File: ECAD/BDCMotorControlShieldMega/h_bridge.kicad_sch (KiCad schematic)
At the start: 23 parts, among them J18 Motor Connector, J19 Limit switch, J8 Limit switch, U14 INA180A1, U7 DRV8870DDA

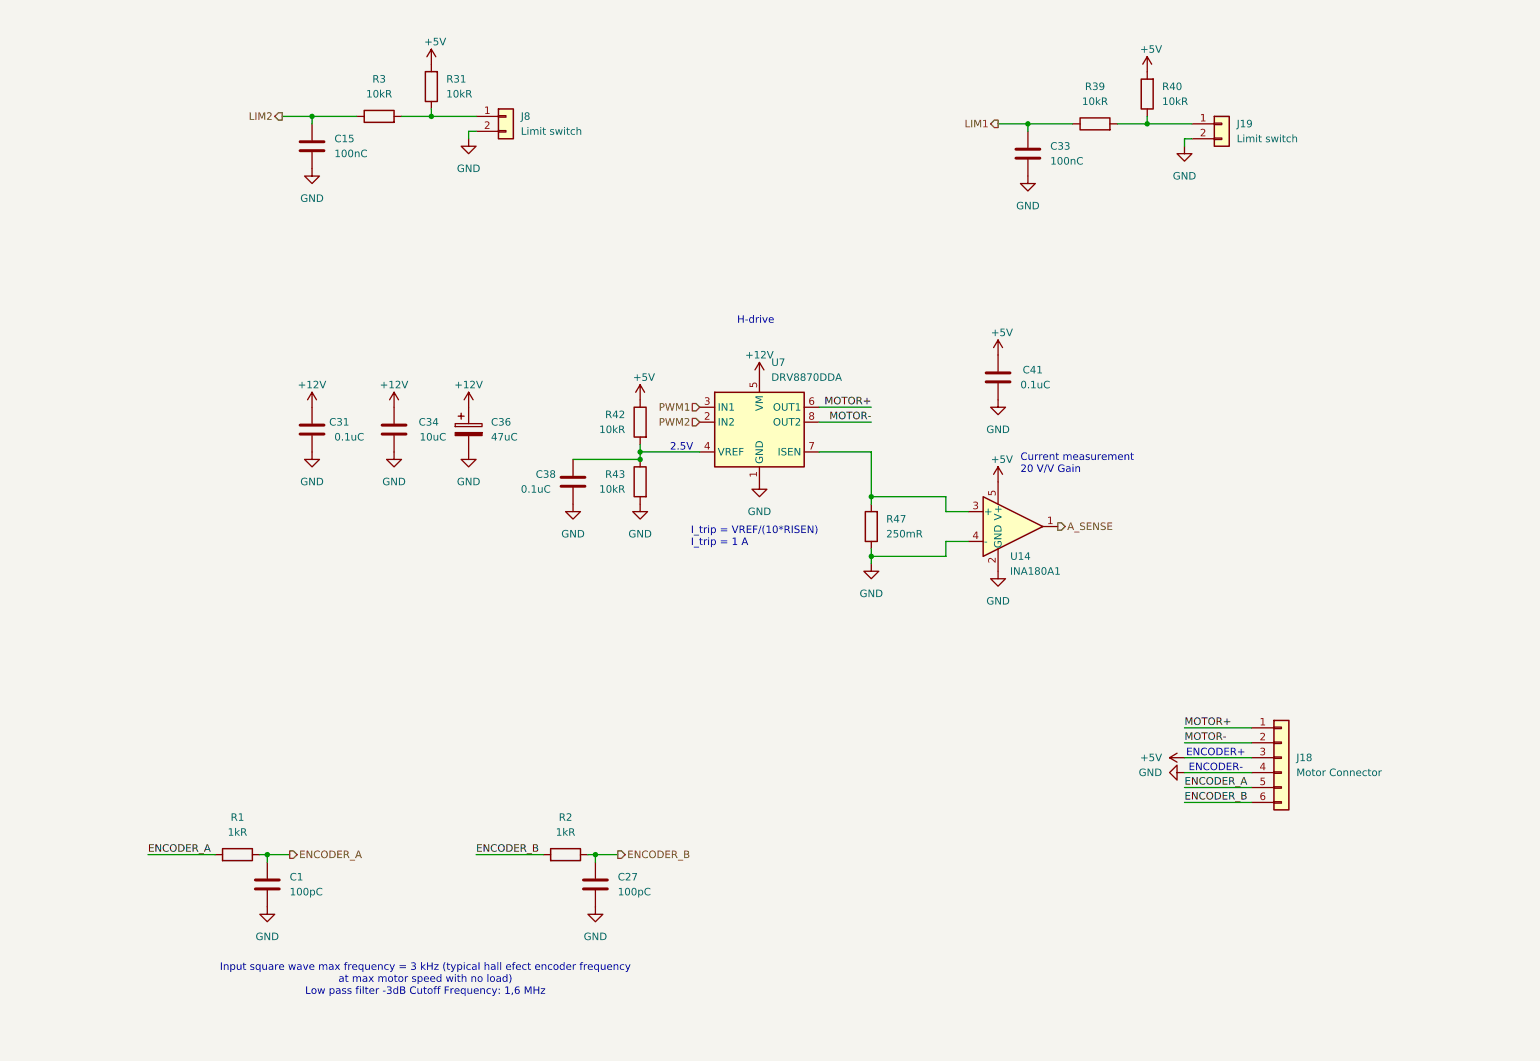
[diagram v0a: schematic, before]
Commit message: Progressed ECAD.
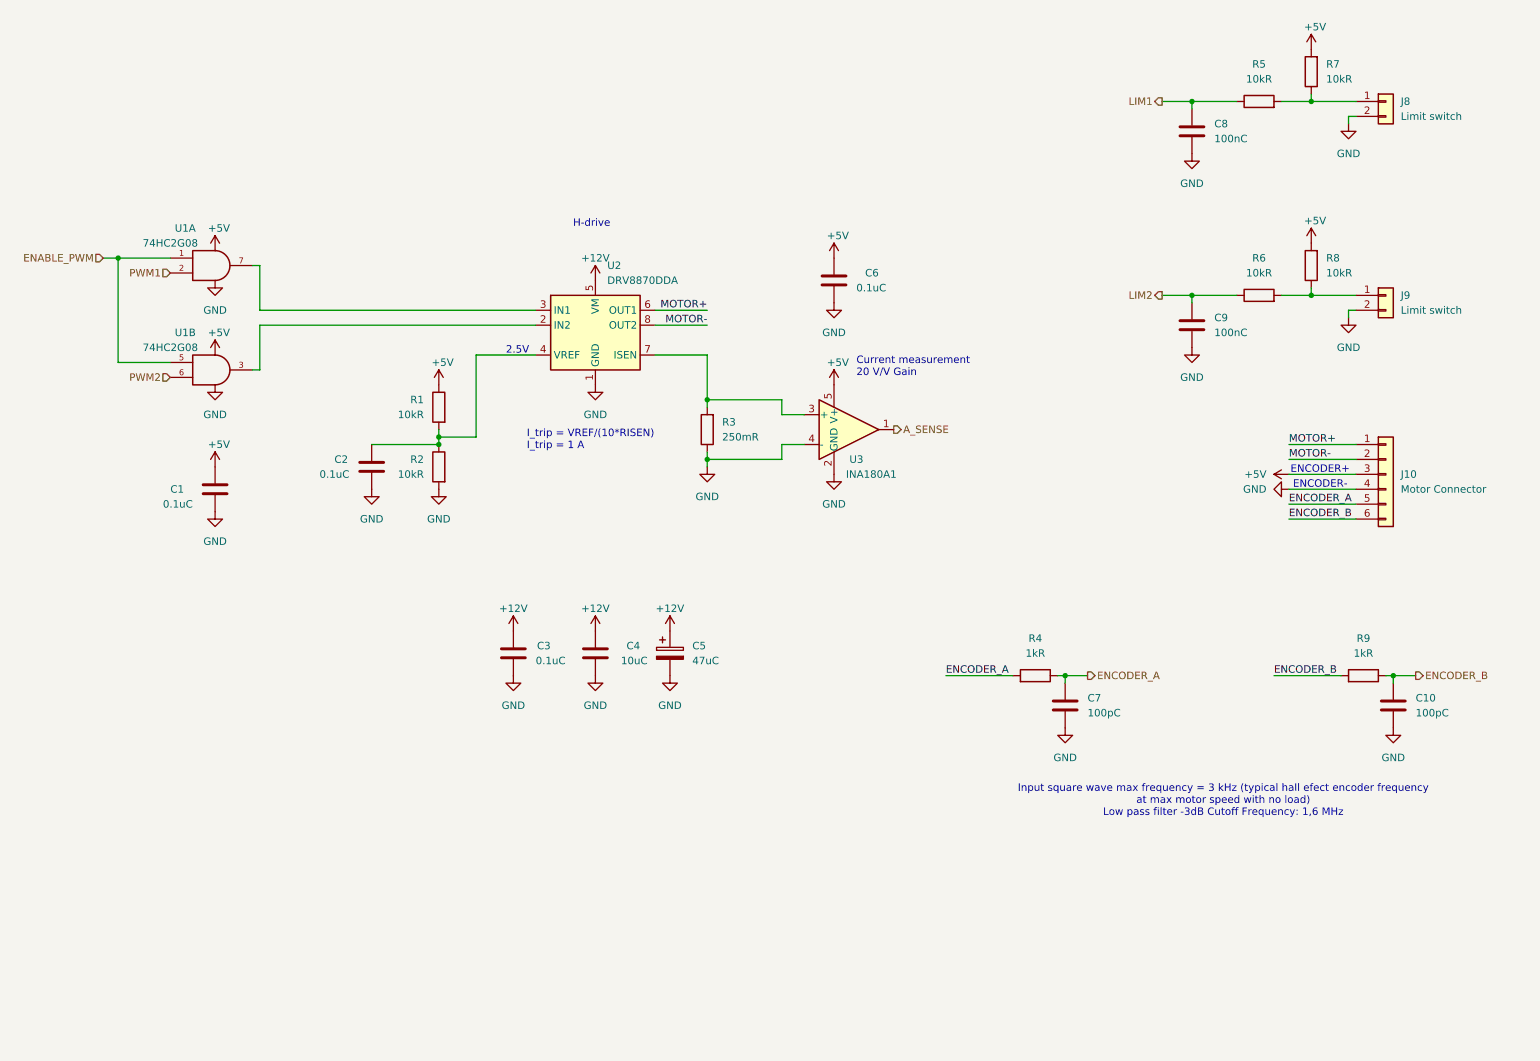
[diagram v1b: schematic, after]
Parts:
- added C1: 0.1uC, Capacitor_SMD:C_0805_2012Metric_Pad1.18x1.45mm_HandSolder, symbol Device:C
- added U1: 74HC2G08, Package_SO:TSSOP-8_3x3mm_P0.65mm, symbol 74xGxx:74LVC2G08
- renumbered C27 to C10, C38 to C2, C31 to C3, C34 to C4, C36 to C5, C41 to C6, C1 to C7, C33 to C8, C15 to C9, J18 to J10, J19 to J8, J8 to J9, R42 to R1, R43 to R2, R47 to R3, R1 to R4, R39 to R5, R3 to R6, R40 to R7, R31 to R8, R2 to R9, U7 to U2, U14 to U3
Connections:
- net +5V: now also C1.1, U1.8 (VCC), U1.8 (VCC)
- net GND: now also C1.2, U1.4 (GND), U1.4 (GND)
- net PWM1: now also U1.2; no longer U2.3 (IN1)
- net PWM2: now also U1.6; no longer U2.2 (IN2)
- new net: U1.3, U2.2 (IN2)
- new net: U1.7, U2.3 (IN1)
- new net ENABLE_PWM: U1.1, U1.5
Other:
- moved on the sheet: C10, C2, C3, C4, C5, C6, C7, C8, C9, J10, J8, J9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

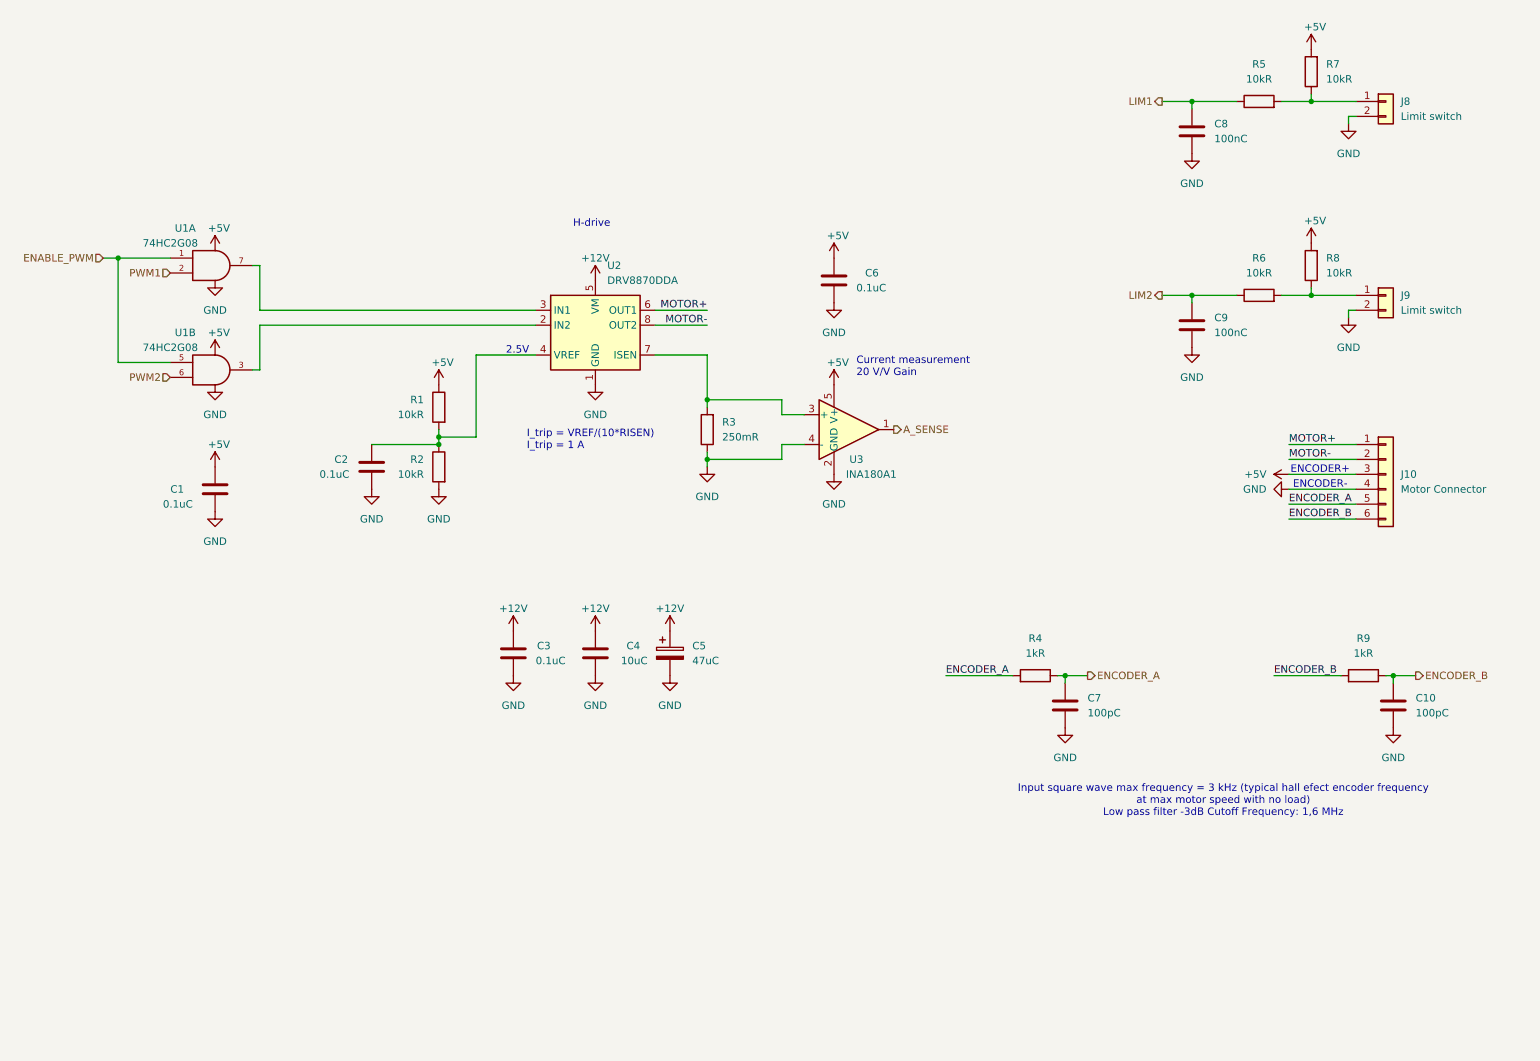
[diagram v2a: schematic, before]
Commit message: Progressed ECAD.
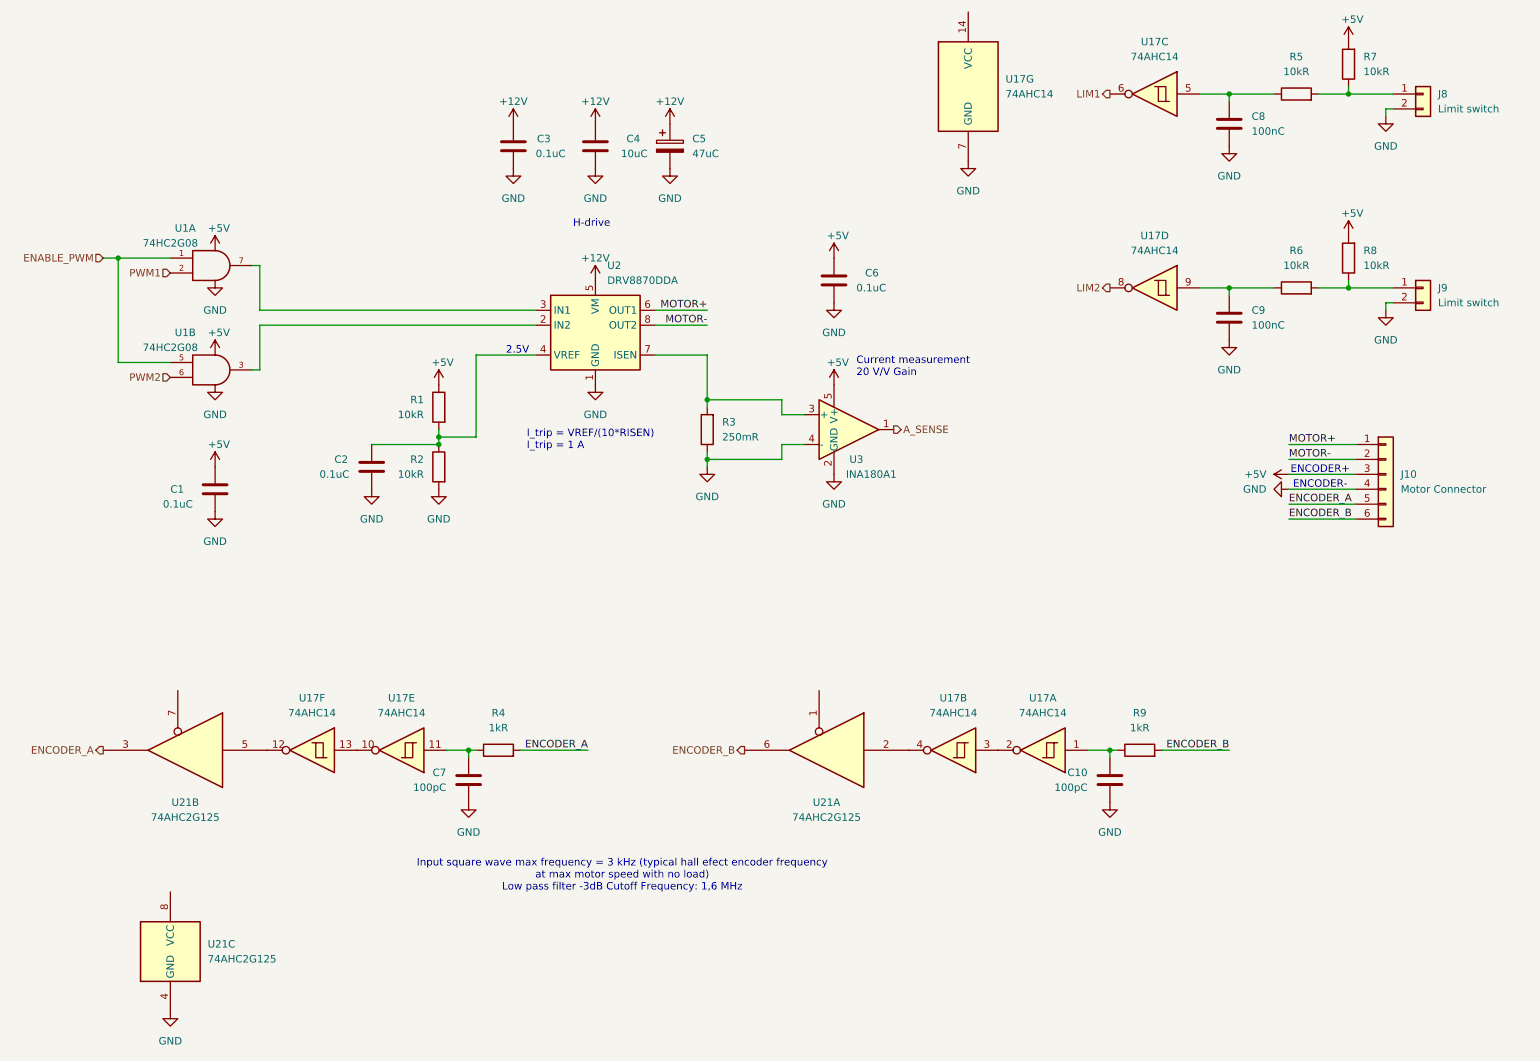
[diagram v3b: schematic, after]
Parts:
- added U17: 74AHC14, Package_SO:TSSOP-14_4.4x5mm_P0.65mm, symbol 74xx:74HC14
- added U21: 74AHC2G125, Package_SO:TSSOP-8_3x3mm_P0.65mm, symbol 74xGxx:74AUC2G125
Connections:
- net ENCODER_A: now also U21.3; no longer C7.1, R4.1
- net ENCODER_B: now also U21.6; no longer C10.1, R9.1
- net GND: now also U17.7 (GND), U21.4 (GND)
- net LIM1: now also U17.6; no longer C8.1, R5.1
- net LIM2: now also U17.8; no longer C9.1, R6.1
- new net: C8.1, R5.1, U17.5
- new net: C10.1, R9.1, U17.1
- new net: U17.4, U21.2
- new net: U17.12, U21.5
- new net: C9.1, R6.1, U17.9
- new net: U17.10, U17.13
- new net: C7.1, R4.1, U17.11
- new net: U17.2, U17.3
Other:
- moved on the sheet: C10, C3, C4, C5, C7, C8, C9, J8, J9, R4, R5, R6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
